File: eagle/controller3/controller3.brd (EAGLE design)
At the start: 55.9 x 50.8 mm, 37 parts, among them J1 FEMALE 2x3, J4 USB-MICROB

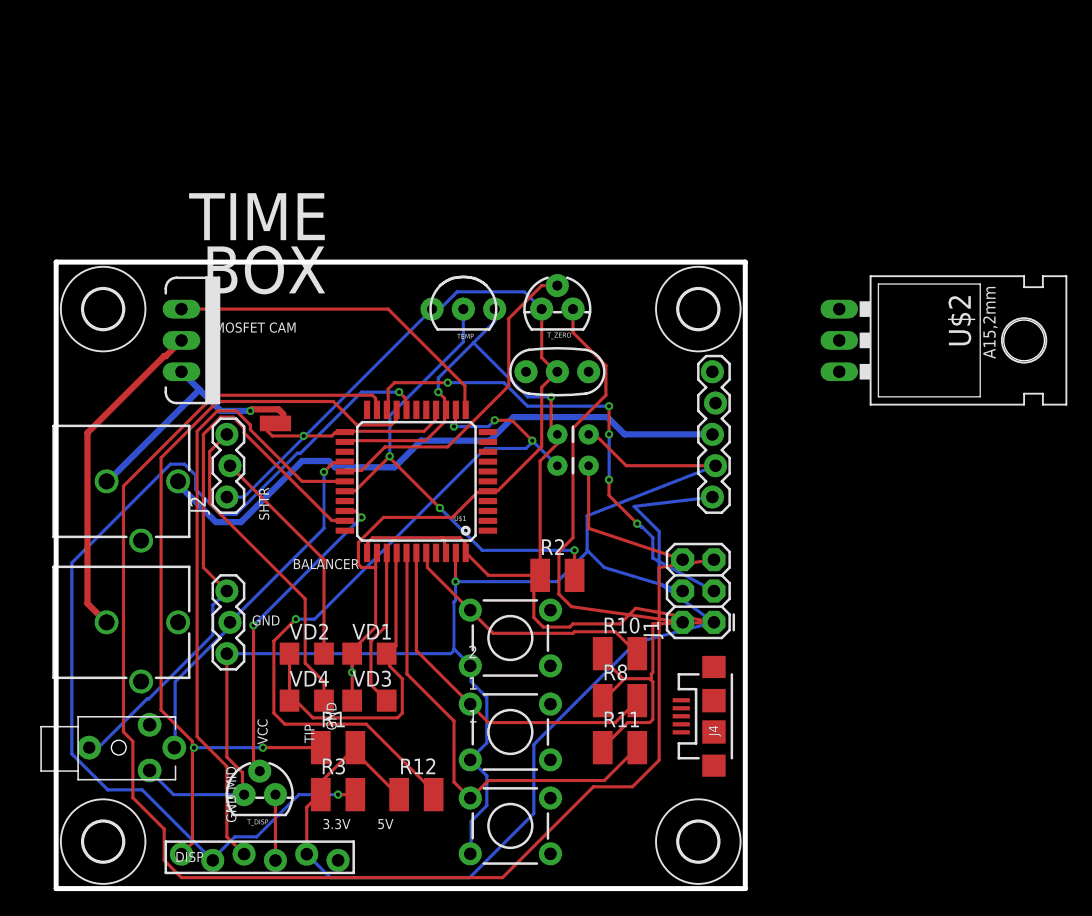
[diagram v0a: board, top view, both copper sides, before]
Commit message: controller3 update eagle files
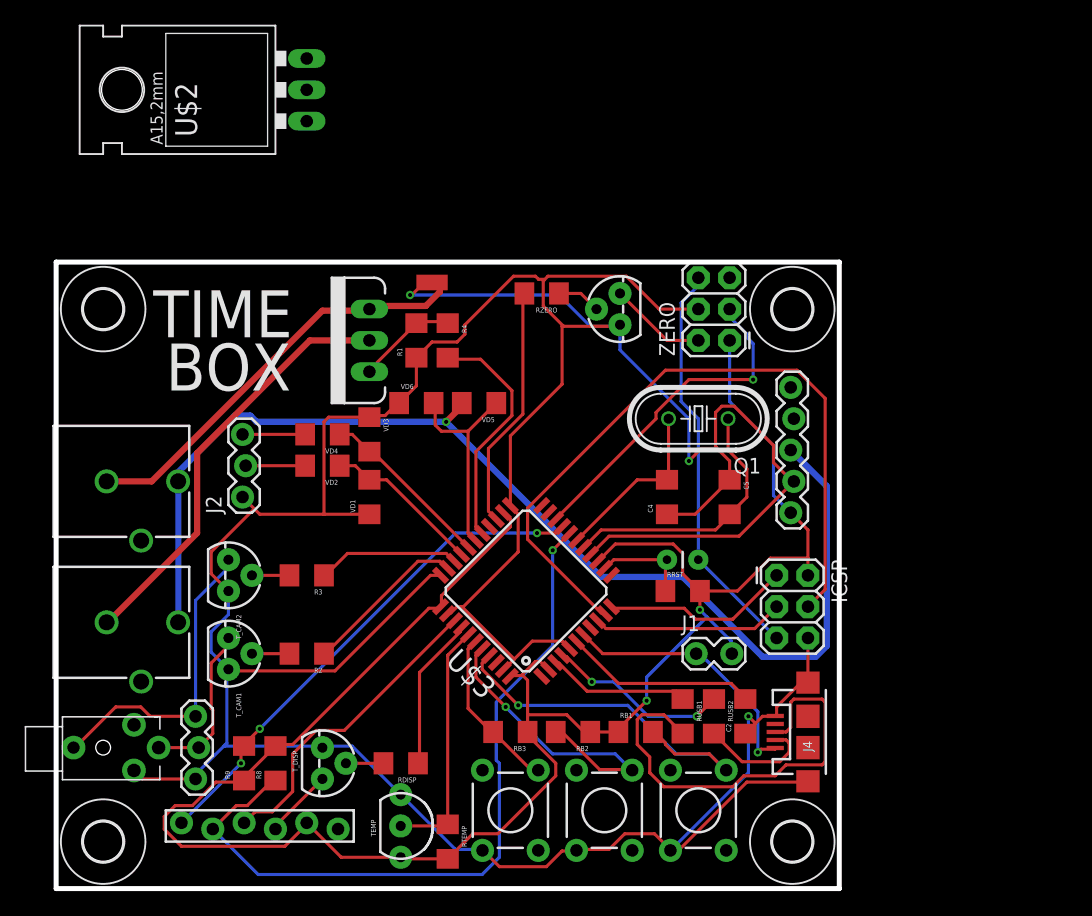
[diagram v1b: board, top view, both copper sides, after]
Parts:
- removed C3: 100nF, SparkFun-Passives:CAP-PTH-SMALL
- removed R10, R11, R12: (no value), adafruit:R3225
- removed RES: (no value), SparkFun-FreqCtrl:RESONATOR-PTH
- removed U$1: ATMEGA32U4TQFP, SparkFun-Retired:SPARKFUN-DIGITALIC_TQFP44
- added C2: (no value), SparkFun-Capacitors:1206
- added C4, C5, R4, R9, RB1, RB2, RB3, RDISP, RRST, RTEMP, RUSB1, RUSB2, RZERO, VD5, VD6: (no value), SparkFun-Passives:1206
- added ICSP, ZERO: (no value), SparkFun-Connectors:2X3
- added Q1: (no value), adafruit:HC49U70
- added T_CAM1, T_CAM2: (no value), SparkFun-DiscreteSemi:TO-92
- added U$3: ATMEGA32U4-AU, adafruit:TQFP44
- J1: value FEMALE 2x3 -> (none); device SparkFun-Connectors:2X3 -> SparkFun-Connectors:1X02_LOCK
- R1, R2, R3, R8: device adafruit:R3225 -> SparkFun-Passives:1206
- VD1, VD2, VD3, VD4: device adafruit:R3216 -> SparkFun-Passives:1206
- moved U$2 54.7 mm to (16.5, 64.8), turned to 90 degrees
- moved TEMP 42.2 mm to (27.9, 5.08), turned to 270 degrees
- moved R1 33.6 mm to (29.2, 44.5), turned to 90 degrees
- moved R8 28.4 mm to (17.8, 10.2), turned to 90 degrees
- moved VD4 21.6 mm to (21.6, 36.8), turned to 180 degrees
- moved VD3 21.6 mm to (25.4, 36.8), turned to 270 degrees
- moved R2 21.3 mm to (20.3, 19.1), turned to 180 degrees
- moved R3 18.0 mm to (20.3, 25.4), turned to 180 degrees
- moved SH 17.1 mm to (30.5, 49.1)
- moved BTN_UP 15.3 mm to (52.1, 6.35), turned to 90 degrees
- moved VD2 15.3 mm to (21.6, 34.3), turned to 180 degrees
- moved MOSFET_CAM 15.2 mm to (25.4, 44.5), turned to 90 degrees
- moved BTN_X 14.0 mm to (36.8, 6.35), turned to 90 degrees
- moved VD1 12.7 mm to (25.4, 31.8), turned to 90 degrees
- moved C1 11.7 mm to (52.1, 26.7)
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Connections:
- removed net CAM_VCC: PWR_CAM.PWR
- removed net EXT_EN: U$1.30
- removed net N$7: J4.GND, J4.MT1, J4.MT2
- new net MISO: ICSP.1, U$3.11
- new net MOSI: ICSP.4, U$3.10
- new net N$12: RZERO.1, T_ZERO.2
- new net N$13: RDISP.2, T_DISP.2
- new net N$14: J4.D+, RUSB1.2
- new net N$15: J4.D-, RUSB2.2
- new net N$16: J3.TIP, SHTR.2, T_CAM1.1
- new net N$17: J3.SHIELD, SHTR.3, T_CAM2.1
- new net N$18: R2.2, T_CAM1.2
- new net N$19: R3.2, T_CAM2.2
- new net N$20: C2.2, U$3.6
- new net N$21: MOSFET_CAM.1, R1.2, R4.1
- new net N$23: U$3.26
- new net N$24: U$3.22
- new net N$28: U$3.12
- new net SCK: ICSP.3, U$3.9
- new net VD_DIRECT: U$3.28, VD5.1, VD6.2
- net BATT_VCC: now also PWR_CAM.PWR, VD5.2
- net BTN1: now also RB1.2, U$3.41; no longer R11.2, U$1.38
- net BTN2: now also RB2.2, U$3.40; no longer R8.2, U$1.39
- net BTN3: now also RB3.2, U$3.39; no longer R10.2, U$1.40
- net CAM1: now also R2.1, U$3.32; no longer J3.SHIELD, SHTR.3, U$1.32
- net CAM2: now also R3.1, U$3.31; no longer J3.TIP, SHTR.2, U$1.26
- net CAM_EN: now also R4.2, U$3.27; no longer MOSFET_CAM.1, U$1.12
- net CELL1: now also U$3.29, VD3.2; no longer U$1.37, VD1.2, VD2.1
- net CELL2: now also U$3.30, VD1.2, VD2.1; no longer U$1.36, VD3.2
- net DISP_EN: now also RDISP.1, U$3.37; no longer T_DISP.2, U$1.31
- net DISP_RST: now also U$3.36; no longer U$1.28
- net GND: now also BTN_DW.1, BTN_UP.1, BTN_X.1, C2.1, C4.1, C5.1, ICSP.6, J4.GND, J4.MT1, J4.MT2, R1.1, T_CAM1.3, T_CAM2.3, U$3.15, U$3.23, U$3.33, U$3.35, U$3.43, U$3.5, VD6.1, ZERO.4; no longer BTN_DW.2, BTN_UP.2, BTN_X.2, C3.1, J1.4, RES.2, U$1.15, U$1.23, U$1.35, U$1.43, U$1.5
- net N$1: now also RRST.1, U$3.13; no longer R12.2, U$1.13
- net N$10: now also ZERO.2; no longer J1.2
- net N$11: now also J1.1, U$3.7; no longer U$1.7
- net N$4: now also RUSB1.1, U$3.3; no longer J4.D-, U$1.3
- net N$5: now also RUSB2.1, U$3.4; no longer J4.D+, U$1.4
- net N$8: now also C4.2, Q1.2, U$3.17; no longer RES.3
- net N$9: now also C5.2, Q1.1, U$3.16; no longer RES.1
- net RST: now also ICSP.5, ZERO.6; no longer J1.6
- net RX: now also U$3.20, ZERO.3; no longer J1.3, U$1.20
- net SCL: now also R8.1, U$3.18; no longer R3.2, U$1.18
- net SDA: now also R9.2, U$3.19; no longer R1.1, U$1.19
- net TEMP: now also RTEMP.1, U$3.38; no longer R2.2, U$1.29
- net TX: now also U$3.21, ZERO.5; no longer J1.5, U$1.21
- net VCC: now also ICSP.2, J1.2, R8.2, R9.1, RB1.1, RB2.1, RB3.1, RRST.2, RTEMP.2, U$3.14, U$3.2, U$3.24, U$3.34, U$3.44, ZERO.1; no longer C3.2, J1.1, R1.2, R10.1, R11.1, R12.1, R2.1, R3.1, R8.1, U$1.14, U$1.24, U$1.34, U$1.42, U$1.44
- net ZERO_EN: now also RZERO.2, U$3.25; no longer T_ZERO.2, U$1.27
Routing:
- net TX: track 121.1 -> 0.00 mm
- net GND: track 208.9 -> 316.2 mm
- net MOSI: track 0.00 -> 58.5 mm
- net N$1: track 61.0 -> 7.89 mm, vias 4 -> 0
- net BATT_VCC: track 49.4 -> 94.4 mm, vias 0 -> 1
- net N$14: track 0.00 -> 36.0 mm
- net CAM1: track 47.1 -> 13.3 mm
- net N$10: track 36.3 -> 7.93 mm
- net DISP_RST: track 51.1 -> 25.6 mm
- net N$17: track 0.00 -> 25.4 mm
- net SDA: track 66.7 -> 41.6 mm, vias 2 -> 3
- net VCC: track 186.0 -> 161.2 mm
- net N$9: track 0.00 -> 22.0 mm
- net N$11: track 0.00 -> 21.6 mm, vias 0 -> 1
- net SCL: track 82.4 -> 61.0 mm, vias 2 -> 1
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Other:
- board size 55.9 x 50.8 mm -> 63.5 x 50.8 mm
- board text removed: "1"
- board text removed: "2"
- board text removed: "3.3V"
- board text removed: "5V"
- board text removed: "BALANCER"
- board text removed: "DISP"
- board text removed: "GND"
- board text removed: "MID"
- board text removed: "MOSFET CAM"
- board text removed: "SHTR"
- board text removed: "TIP"
- board text removed: "VCC"
